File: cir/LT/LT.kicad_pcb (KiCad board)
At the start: 2 copper layers, 66.7 x 23.3 mm, 24 parts, among them J1 Conn_01x04_Socket, J2 Conn_01x04_Socket, J3 Conn_01x02_Socket, U1 LBR-127HLD, U2 74HC7014, U4 LBR-127HLD, U5 LBR-127HLD, U6 LBR-127HLD

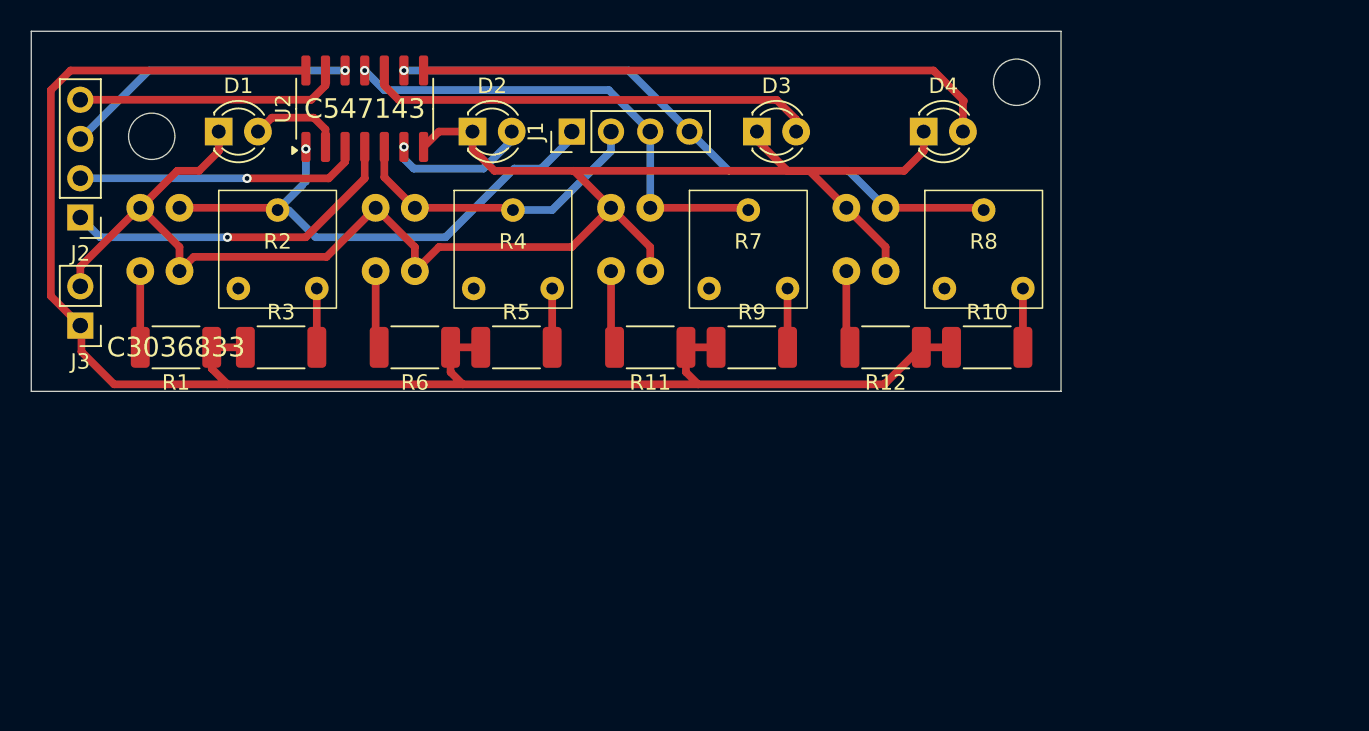
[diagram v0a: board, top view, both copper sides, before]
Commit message: u
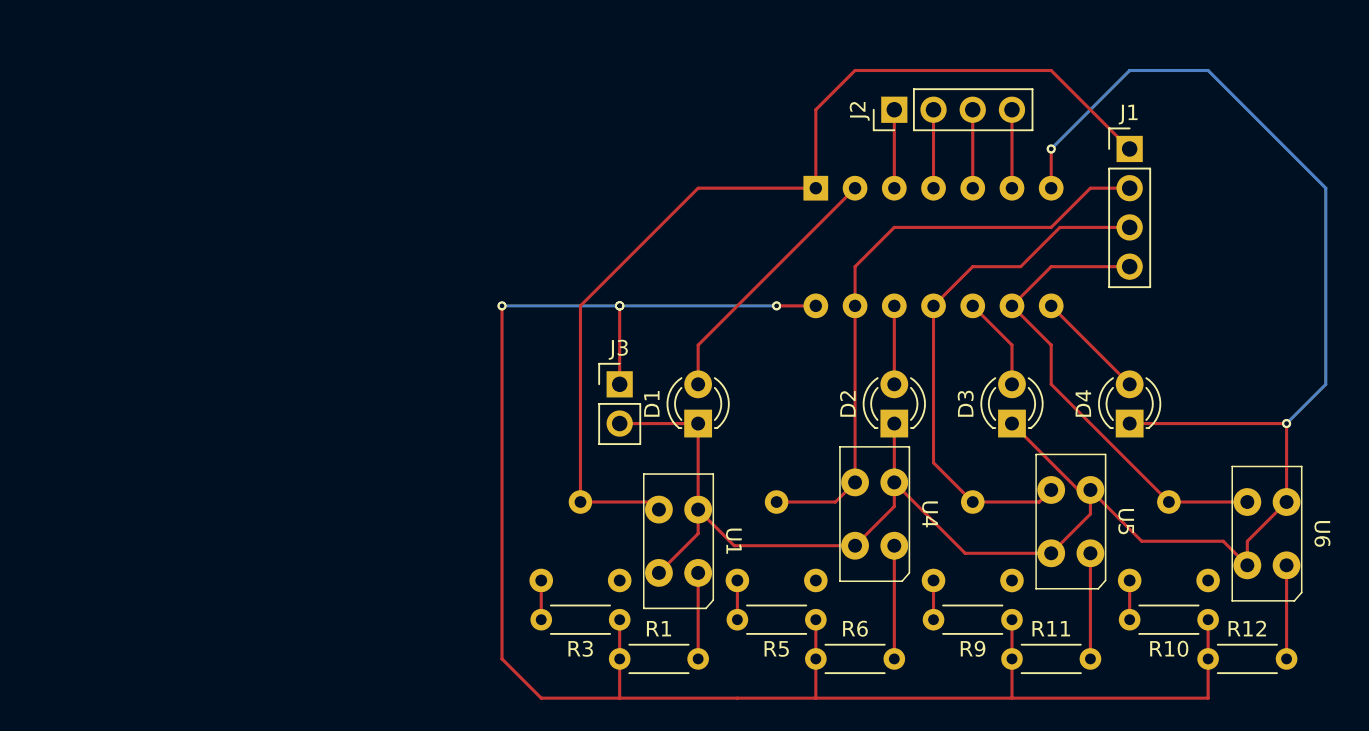
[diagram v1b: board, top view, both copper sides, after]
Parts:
- R1, R10, R11, R12, R3, R5, R6, R9: footprint Resistor_SMD:R_2010_5025Metric -> Resistor_THT:R_Axial_DIN0204_L3.6mm_D1.6mm_P5.08mm_Horizontal
- R2, R4, R7, R8: moved to B.Cu
- U1, U4, U5, U6: moved to F.Cu
- U2: footprint Package_SO:SOIC-14_3.9x8.7mm_P1.27mm -> Package_DIP:DIP-14_W7.62mm_Socket; moved to B.Cu
- moved J2 53.2 mm to (68.6, 17.8), turned to 90 degrees
- moved U1 38.9 mm to (54.6, 45.7)
- moved D1 36.3 mm to (55.9, 38.1), turned to 90 degrees
- moved J1 36.1 mm to (83.8, 20.3), turned to 0 degrees
- moved U4 35.8 mm to (67.3, 44.0)
- moved J3 35.1 mm to (50.8, 35.6), turned to 0 degrees
- moved R1 35.1 mm to (50.8, 53.3), turned to 0 degrees
- moved U5 33.9 mm to (80.0, 44.5)
- moved D2 33.2 mm to (68.6, 38.1), turned to 90 degrees
- moved R6 32.9 mm to (63.5, 53.3), turned to 0 degrees
- moved U6 32.2 mm to (92.7, 45.2)
- moved R11 30.9 mm to (76.2, 53.3), turned to 0 degrees
- moved U2 29.7 mm to (63.5, 22.9), turned to -90 degrees
- moved R12 29.0 mm to (88.9, 53.3), turned to 0 degrees
- moved R3 28.1 mm to (50.8, 50.8), turned to 180 degrees
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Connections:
- net S1 renamed Net-(J1-Pin_1)
- net S3 renamed Net-(J1-Pin_3)
- net S4 renamed Net-(J1-Pin_4)
- J1 pad 2: S2 -> Net-(J1-Pin_2)
- R4 pad 1: S2 -> Net-(J1-Pin_2)
- U2 pad 12: Net-(J2-Pin_3) -> Net-(D2-A)
- U2 pad 13: Net-(J2-Pin_4) -> Net-(J1-Pin_2)
- U2 pad 3: Net-(J2-Pin_2) -> Net-(J2-Pin_1)
- U2 pad 4: Net-(J2-Pin_1) -> Net-(J2-Pin_2)
- U2 pad 5: S2 -> Net-(J2-Pin_3)
- U2 pad 6: Net-(D2-A) -> Net-(J2-Pin_4)
- U4 pad 4: S2 -> Net-(J1-Pin_2)
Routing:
- net Net-(J1-Pin_2): track 0.00 -> 39.5 mm
- net Net-(J1-Pin_1): track 34.0 -> 64.9 mm, vias 1 -> 0
- net Net-(D4-A): track 37.8 -> 7.18 mm
- net Net-(D3-A): track 29.3 -> 6.13 mm
- net GND: track 111.9 -> 134.0 mm, vias 0 -> 2
- net S2: track 20.4 -> 0.00 mm
- net Net-(J2-Pin_1): track 22.6 -> 5.08 mm, vias 1 -> 0
- net Net-(J2-Pin_3): track 19.0 -> 5.08 mm, vias 1 -> 0
- net Net-(J2-Pin_2): track 18.6 -> 5.08 mm, vias 1 -> 0
- net Net-(J2-Pin_4): track 17.2 -> 5.08 mm
- net Net-(D1-A): track 6.20 -> 16.9 mm
- net Net-(J1-Pin_4): track 41.3 -> 30.7 mm, vias 1 -> 0
- net +5V: track 107.3 -> 115.4 mm, vias 0 -> 4
- net Net-(D2-A): track 9.46 -> 5.08 mm, vias 1 -> 0
- net Net-(J1-Pin_3): track 31.5 -> 34.0 mm, vias 1 -> 0
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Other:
- board outline removed
